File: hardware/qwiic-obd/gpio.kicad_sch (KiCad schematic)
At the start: 24 parts, among them SW401 SW_Push, U401 TCA9534, U402 MCP3423, U403 TCA9534, U404 ADM6320BX33ARJZ-R7, U405 TCA9534

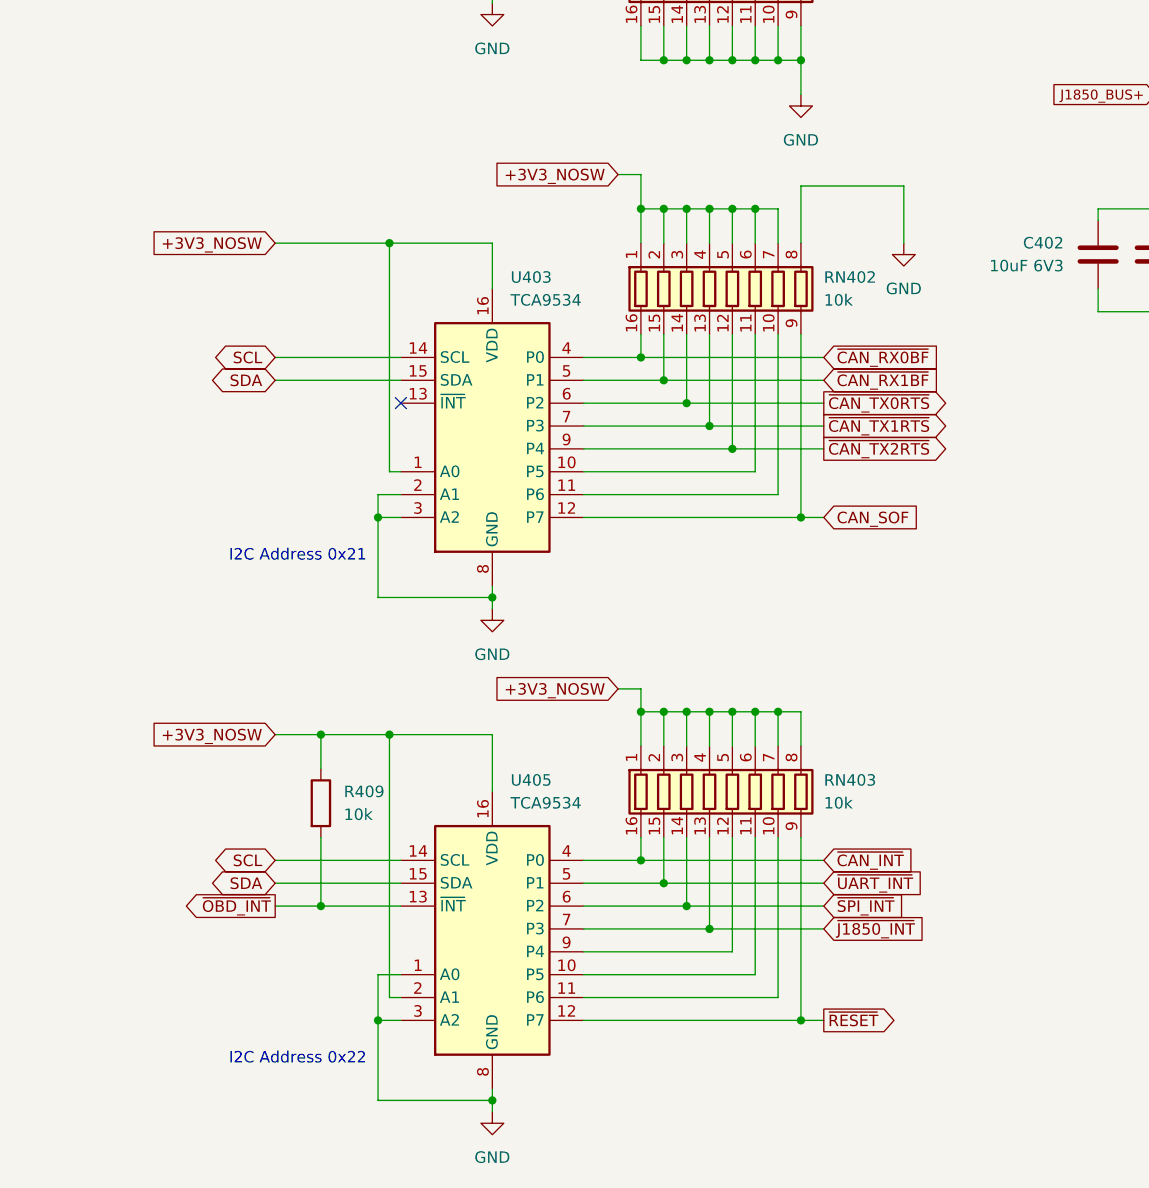
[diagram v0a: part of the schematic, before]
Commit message: OK, layout v1 complete
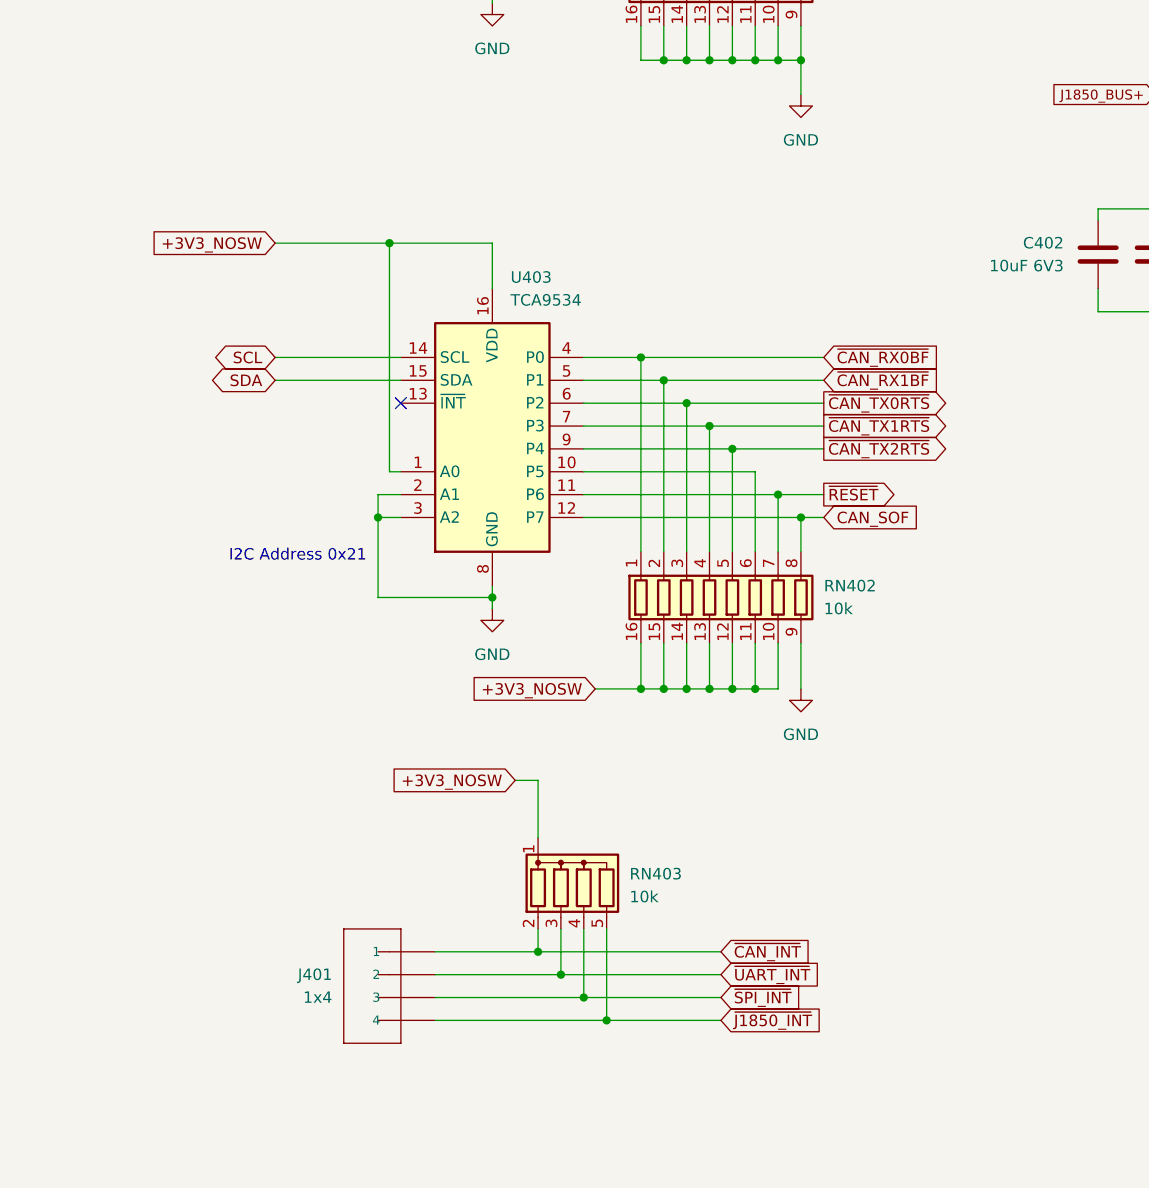
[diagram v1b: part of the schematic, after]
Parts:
- removed R409: 10k, Resistor_SMD:R_0805_2012Metric_Pad1.20x1.40mm_HandSolder, symbol Device:R
- removed RN403: 10k, UltraLibrarian:742C163103JP, symbol Device:R_Pack08
- removed U405: TCA9534, Package_SO:TSSOP-16_4.4x5mm_P0.65mm, symbol Interface_Expansion:TCA9534
- added J401: 1x4, Connector_PinSocket_2.54mm:PinSocket_1x04_P2.54mm_Vertical, symbol SparkFun-Connectors:M04JST-PTH
- added RN403: 10k, Resistor_THT:R_Array_SIP5, symbol Device:R_Network04
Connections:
- net +3V3_NOSW: now also RN402.10 (R7.2), RN402.11 (R6.2), RN402.12 (R5.2), RN402.13 (R4.2), RN402.14 (R3.2), RN402.15 (R2.2), RN402.16 (R1.2), RN403.1 (common); no longer RN402.1 (R1.1), RN402.2 (R2.1), RN402.3 (R3.1), RN402.4 (R4.1), RN402.5 (R5.1), RN402.6 (R6.1), RN402.7 (R7.1)
- net CAN_SOF: now also RN402.8 (R8.1); no longer RN402.9 (R8.2)
- net GND: now also RN402.9 (R8.2); no longer RN402.8 (R8.1)
- net ~{CAN_INT}: now also J401.1, RN403.2 (R1)
- net ~{CAN_RX0BF}: now also RN402.1 (R1.1); no longer RN402.16 (R1.2)
- net ~{CAN_RX1BF}: now also RN402.2 (R2.1); no longer RN402.15 (R2.2)
- net ~{CAN_TX0RTS}: now also RN402.3 (R3.1); no longer RN402.14 (R3.2)
- net ~{CAN_TX1RTS}: now also RN402.4 (R4.1); no longer RN402.13 (R4.2)
- net ~{CAN_TX2RTS}: now also RN402.5 (R5.1); no longer RN402.12 (R5.2)
- net ~{J1850_INT}: now also J401.4, RN403.5 (R4)
- net ~{RESET}: now also RN402.7 (R7.1), U403.11 (P6)
- net ~{SPI_INT}: now also J401.3, RN403.4 (R3)
- net ~{UART_INT}: now also J401.2, RN403.3 (R2)
- net at U403.10 (P5): now also RN402.6 (R6.1); no longer RN402.11 (R6.2)
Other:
- note removed: "I2C Address 0x22"
- moved on the sheet: RN402
